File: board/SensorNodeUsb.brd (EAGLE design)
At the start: 73 x 22.2 mm, 18 parts, among them X2 USBPCB

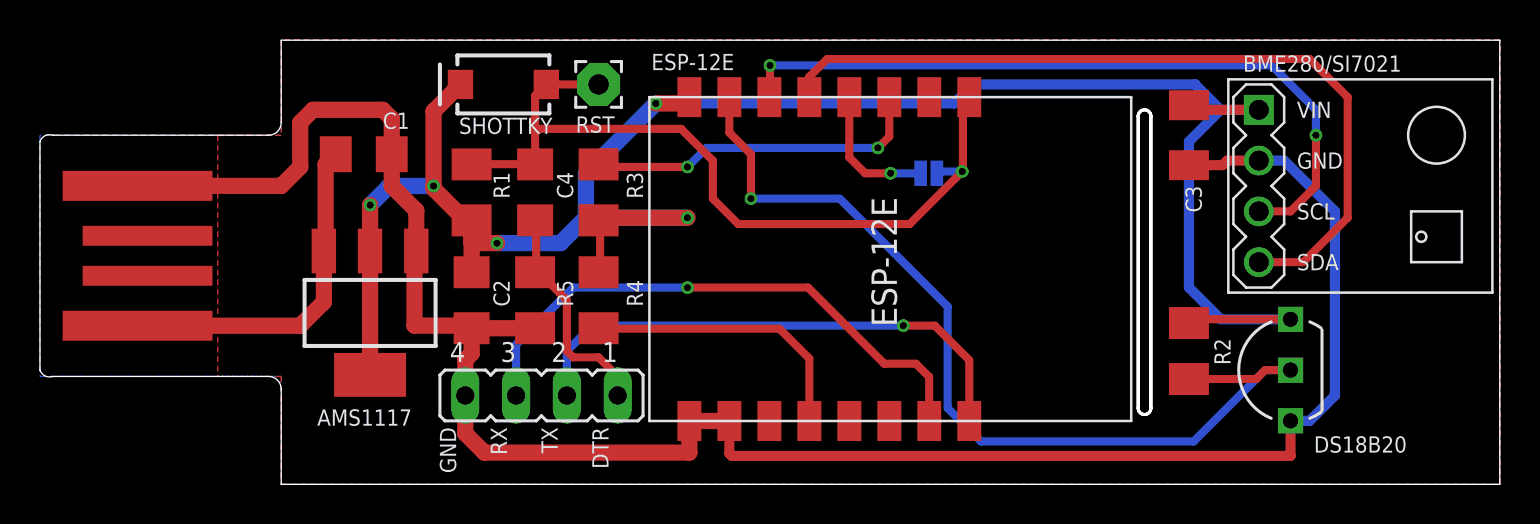
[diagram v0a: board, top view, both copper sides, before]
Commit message: 5-pin programming interface
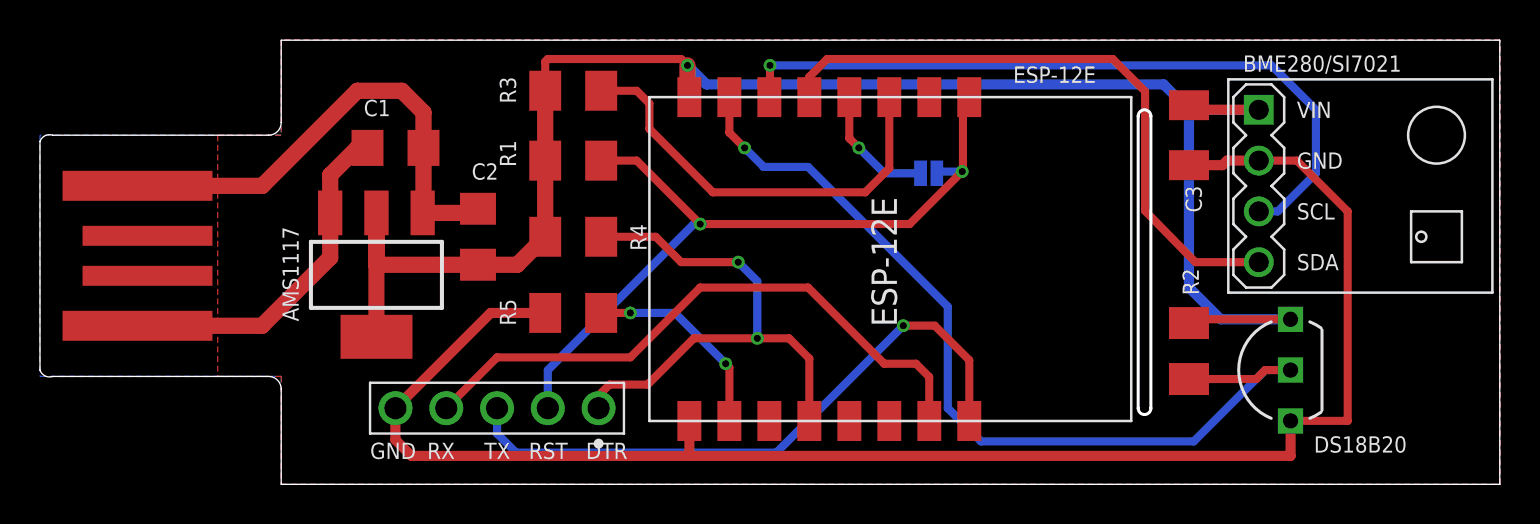
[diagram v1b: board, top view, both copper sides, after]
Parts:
- removed C4: 2.2uF, rcl:C1206
- removed JP2: ISP, jumper:JP4
- removed RST: (no value), wirepad:2,15/1,0
- removed SHOTTKY: Shottky, SparkFun-DiscreteSemi:SMA-DIODE
- added J1: JP5E, thomo:JP5
- R5: value 1k -> 10k
- moved R1 5.32 mm to (26.7, 16.2), turned to 0 degrees
- moved R3 5.24 mm to (26.7, 19.7), turned to 180 degrees
- moved R4 3.42 mm to (26.7, 12.4), turned to 180 degrees
- moved C2 3.19 mm to (21.9, 12.4), turned to 90 degrees
- moved R5 2.01 mm to (26.7, 8.57), turned to 0 degrees
- moved AMS1117 1.93 mm to (16.8, 10.5)
- moved C1 1.62 mm to (17.8, 16.8)
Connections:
- removed net N$1: C4.1, ESP-12E.1, R1.2, RST.1, SHOTTKY.A, WAKEUP.2
- removed net N$4: ESP-12E.12, R4.1
- removed net N$5: C4.2, JP2.1, R5.2
- removed net N$6: ESP-12E.16, JP2.2
- removed net N$7: ESP-12E.15, JP2.3
- new net DTR: ESP-12E.12, J1.1, R4.1
- new net N$9: ESP-12E.10, R5.2
- new net RST: ESP-12E.1, J1.2, R1.2, WAKEUP.2
- new net RX: ESP-12E.15, J1.4
- new net TX: ESP-12E.16, J1.3
- net +3V3: no longer SHOTTKY.C
- net GND: now also J1.5; no longer ESP-12E.10, JP2.4
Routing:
- net N$1: track 40.7 -> 0.00 mm, vias 1 -> 0
- net RST: track 0.00 -> 38.2 mm, vias 0 -> 2
- net TX: track 0.00 -> 31.7 mm, vias 0 -> 1
- net RX: track 0.00 -> 30.7 mm
- net N$7: track 28.4 -> 0.00 mm, vias 1 -> 0
- net DTR: track 0.00 -> 27.5 mm, vias 0 -> 2
- net N$6: track 26.6 -> 0.00 mm, vias 1 -> 0
- net +3V3: track 106.7 -> 88.4 mm, vias 5 -> 1
- net N$4: track 14.3 -> 0.00 mm
- net N$5: track 11.5 -> 0.00 mm
- net N$9: track 0.00 -> 10.2 mm, vias 0 -> 2
- net I2C_SDA: track 40.5 -> 31.6 mm
- net N$3: track 17.2 -> 21.3 mm, vias 2 -> 0
- net GND: track 105.2 -> 106.8 mm
- net DATA_1W: track 47.3 -> 46.0 mm
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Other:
- board text added: "RST"
- board text added: "SensorNode v1.1 ThoMo 07/2019"
- board text removed: "SensorNode ThoMo 04/2019"
